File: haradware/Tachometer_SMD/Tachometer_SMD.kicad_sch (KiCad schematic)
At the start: 14 parts, among them J101 ch1, J103 ch2, J104 Conn_01x04, Q101 NMOS, Q102 NMOS

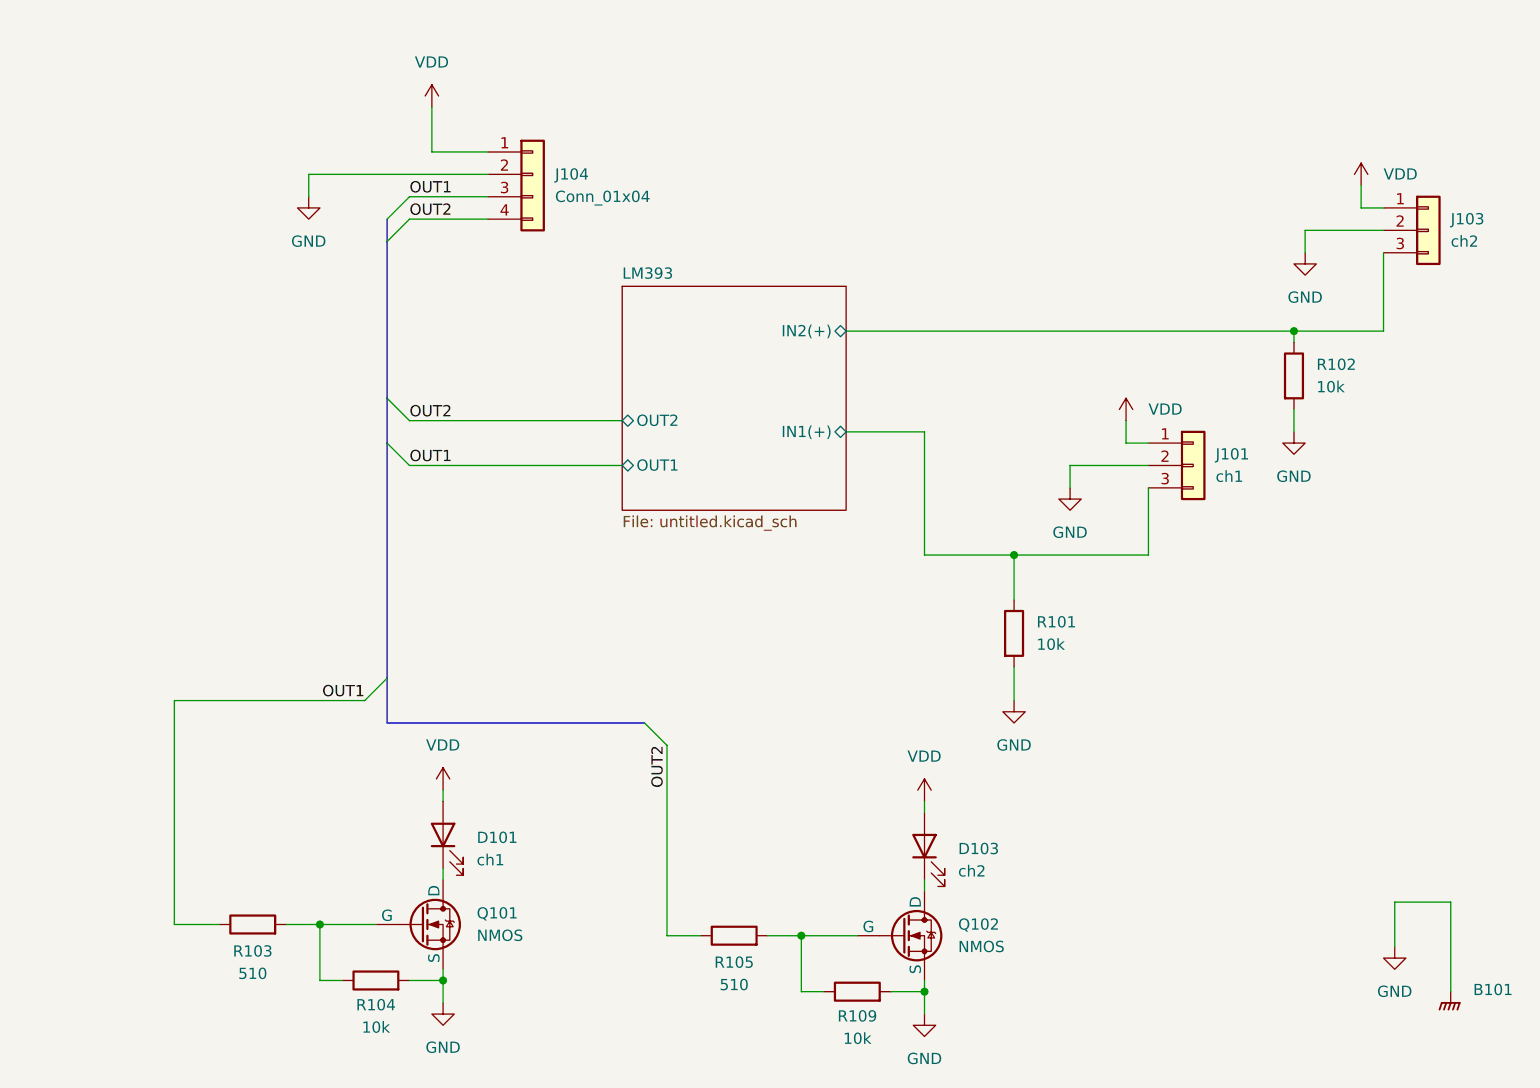
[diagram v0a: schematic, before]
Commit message: ちょっと整理
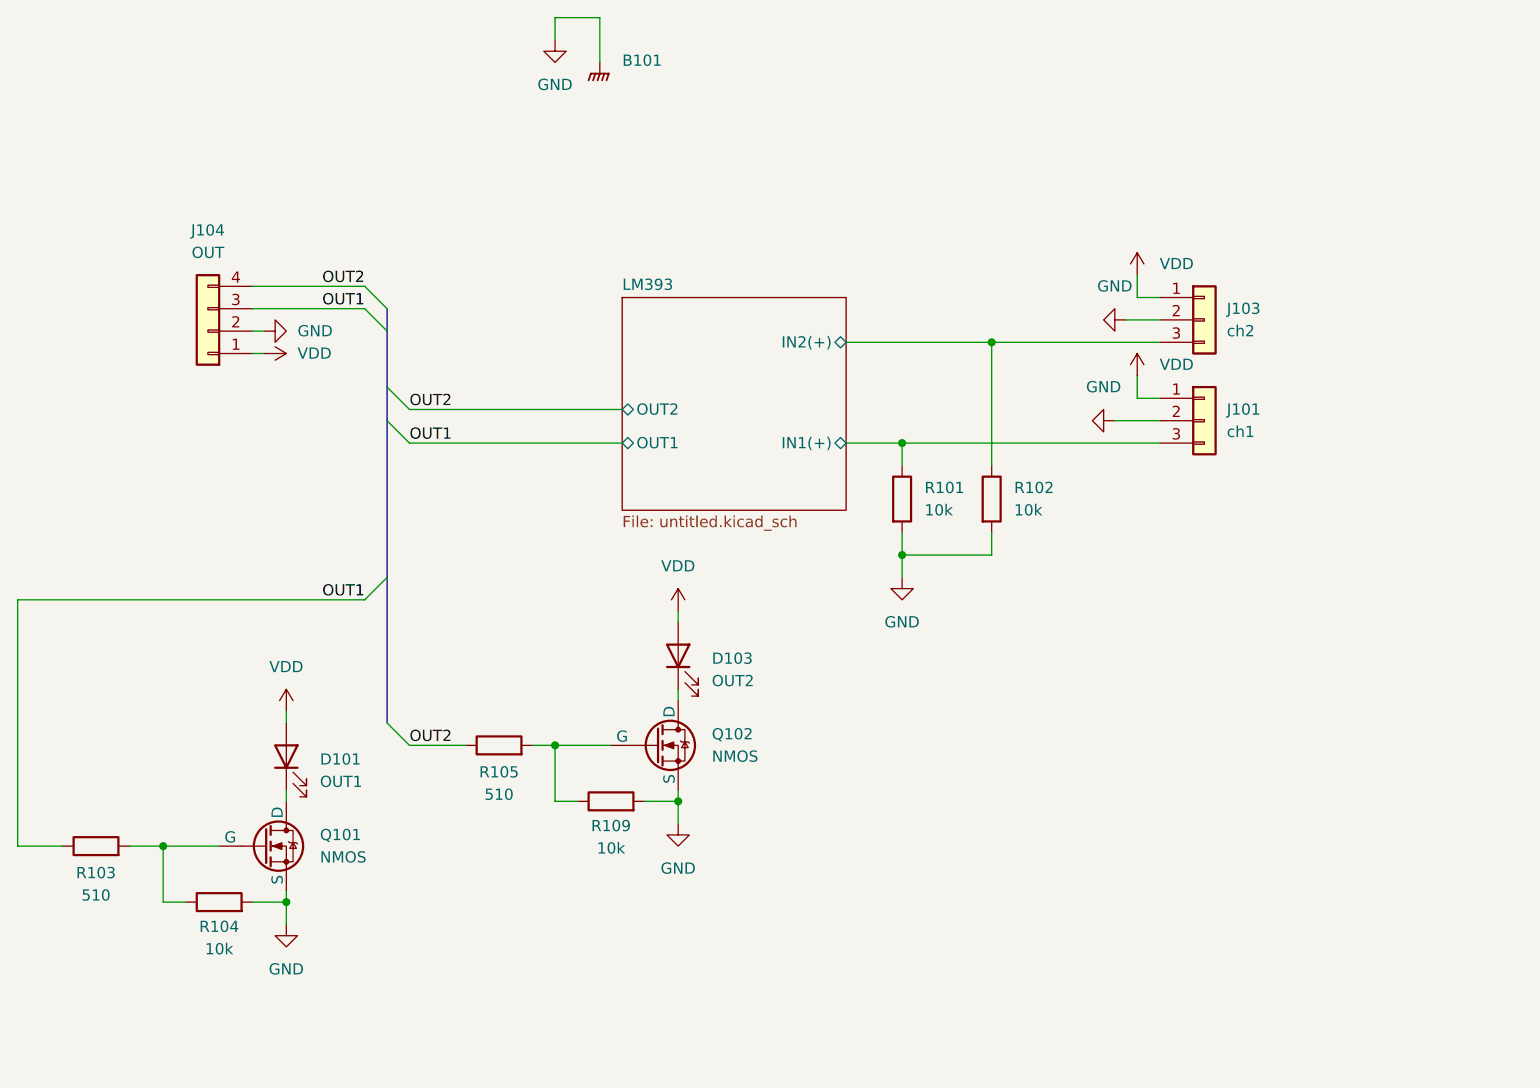
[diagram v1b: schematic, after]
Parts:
- D101: value ch1 -> OUT1
- D103: value ch2 -> OUT2
- J104: value Conn_01x04 -> OUT
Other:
- moved on the sheet: B101, D101, D103, J101, J103, J104, Q101, Q102, R101, R102, R103, R104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
